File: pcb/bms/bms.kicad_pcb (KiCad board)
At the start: 4 copper layers, 80 x 60 mm, 89 parts, among them J12 Taps 6-8, J13 Taps 0-5, J14 USB_B_Micro, J18 SWD, Q1 FCX495TA, Q2 CSD19506KTT, Q3 CSD19506KTT, Q4 ZXMP10A13FTA, Q5 ZXMP10A13FTA, SW1 Boot, SW2 Wake, SW3 NRST, U1 BQ76942PFBR, U2 STM32L422KBTx

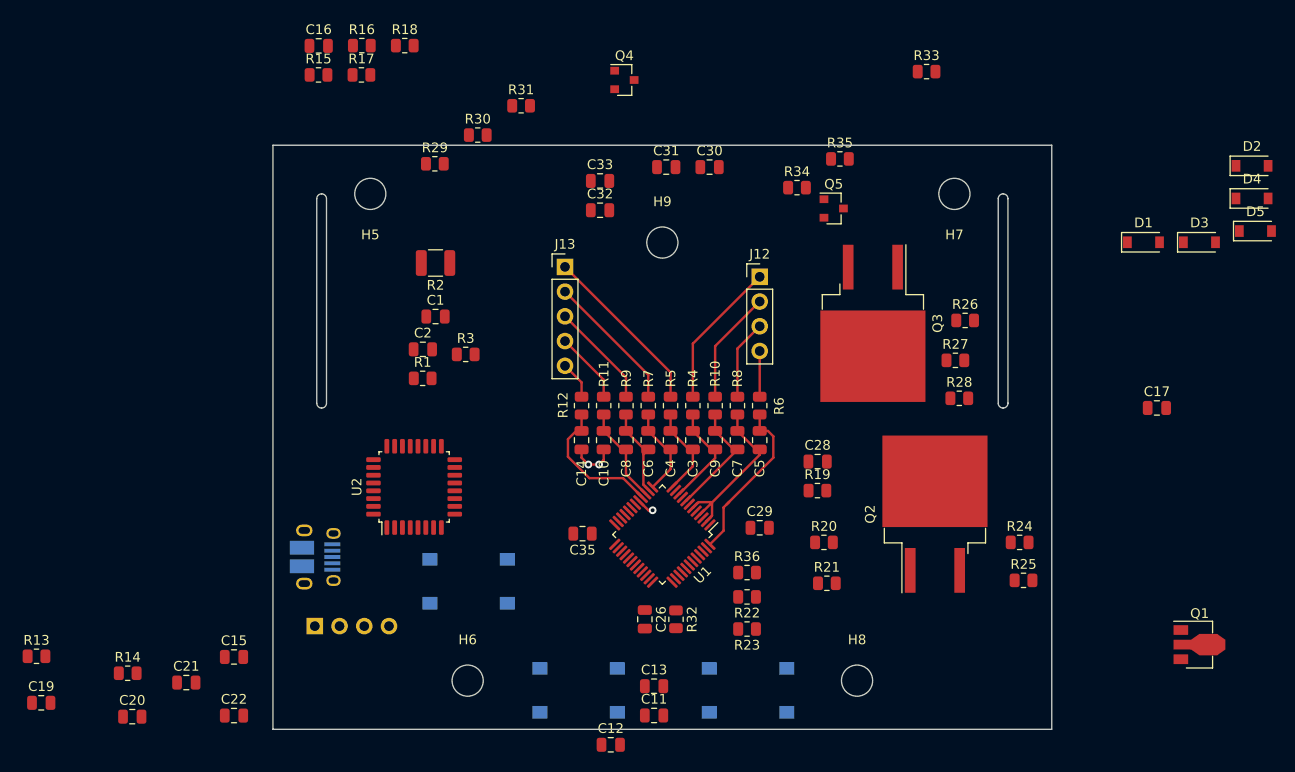
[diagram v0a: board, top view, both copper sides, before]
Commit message: pretty much ready to go
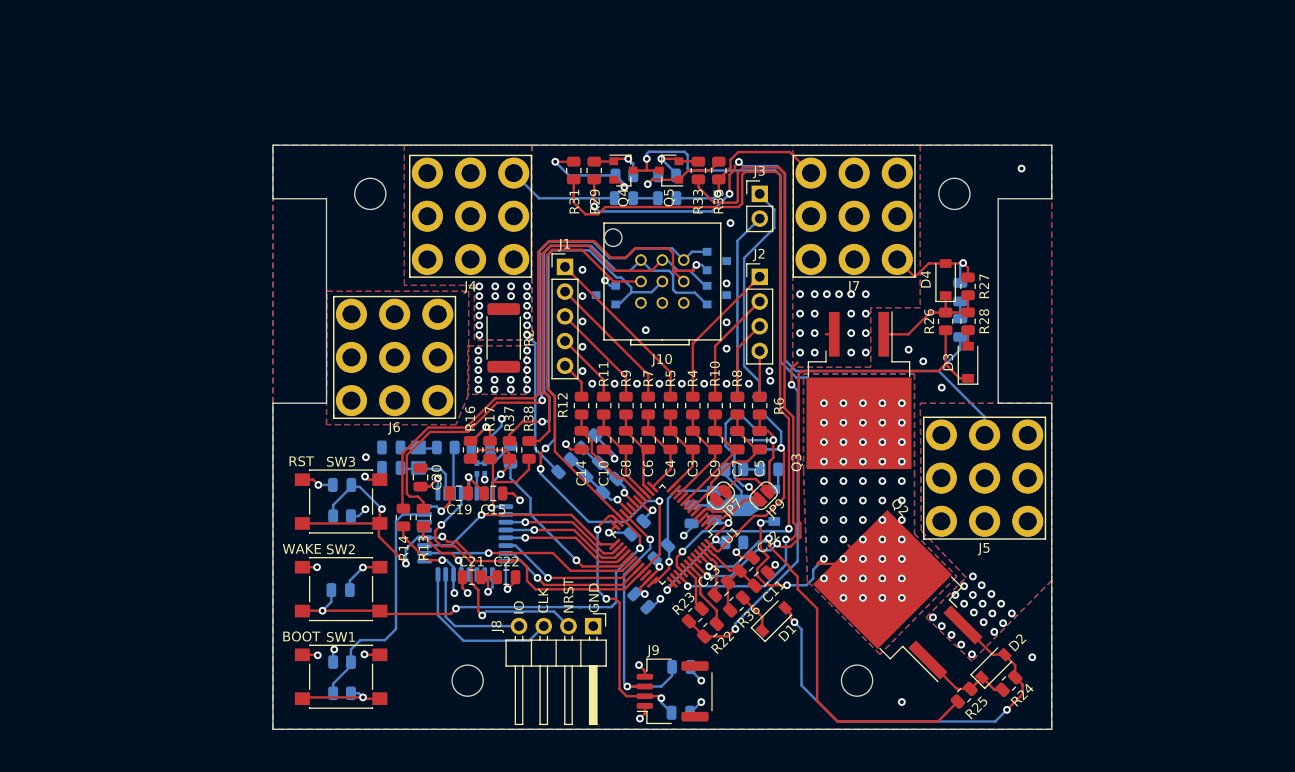
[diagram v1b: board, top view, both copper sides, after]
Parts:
- removed H9: MountingHole, MountingHole:MountingHole_3.2mm_M3
- removed J14: USB_B_Micro, Connect:USB_Micro-B_10103594-0001LF
- removed J18: SWD, Connector_PinHeader_2.54mm:PinHeader_1x04_P2.54mm_Horizontal
- added C18: 100n, Capacitor_SMD:C_0805_2012Metric, B.Cu at (92.0, 113.6)
- added C23: 100n, Capacitor_SMD:C_0805_2012Metric, B.Cu at (91.9, 118.3)
- added C24: 220n, Capacitor_SMD:C_0805_2012Metric, B.Cu at (100.0, 90.3)
- added C25: 220n, Capacitor_SMD:C_0805_2012Metric, B.Cu at (97.7, 90.3)
- added C27: 100n, Capacitor_SMD:C_0805_2012Metric, B.Cu at (71.3, 91.1)
- added C34: 8p, Capacitor_SMD:C_0805_2012Metric, B.Cu at (62.1, 93.2)
- added C36: 8p, Capacitor_SMD:C_0805_2012Metric, B.Cu at (62.1, 91.0)
- added D6: 5.5V, Package_TO_SOT_SMD:SOT-23, B.Cu at (95.6, 71.9)
- added D7: 5.5V, Package_TO_SOT_SMD:SOT-23, B.Cu at (95.6, 75.4)
- added D8: 5.5V, Package_TO_SOT_SMD:SOT-23, B.Cu at (84.2, 75.4)
- added J10: Signals, Connector_Hirose:Hirose_DF62WZ-9P-2.2DSA, F.Cu at (90.0, 74.0)
- added J3: Taps 9-10, Connector_PinHeader_2.54mm:PinHeader_1x02_P2.54mm_Vertical, F.Cu at (100.0, 65.0)
- added J4: Batt- Out, farasis_p10a_pack:74651195R, F.Cu at (70.3, 67.3)
- added J5: Batt+ In, farasis_p10a_pack:74651195R, F.Cu at (123.1, 94.2)
- added J6: Batt- In, farasis_p10a_pack:74651195R, F.Cu at (62.5, 81.8)
- added J7: Batt+ Out, farasis_p10a_pack:74651195R, F.Cu at (109.7, 67.3)
- added J8: SWD, Connector_PinHeader_2.54mm:PinHeader_1x04_P2.54mm_Horizontal, F.Cu at (82.9, 109.4)
- added J9: Thermistors, Connector_JST:JST_NSH_SM04B-NSHSS-TB_1x04-1MP_P1.00mm_Vertical, F.Cu at (88.2, 117.6)
- added JP7: Jumper_NO_Small, Jumper:SolderJumper-2_P1.3mm_Open_RoundedPad1.0x1.5mm, F.Cu at (96.0, 96.0)
- added JP9: Jumper_NO_Small, Jumper:SolderJumper-2_P1.3mm_Open_RoundedPad1.0x1.5mm, F.Cu at (100.4, 96.0)
- added R37: 20, Resistor_SMD:R_0805_2012Metric, F.Cu at (74.3, 91.3)
- added R38: 20, Resistor_SMD:R_0805_2012Metric, F.Cu at (76.3, 91.3)
- added R39: 10k, Resistor_SMD:R_0805_2012Metric, B.Cu at (57.1, 113.1)
- added R40: 20, Resistor_SMD:R_0805_2012Metric, B.Cu at (100.0, 86.8)
- added R41: 20, Resistor_SMD:R_0805_2012Metric, B.Cu at (97.7, 86.8)
- added R42: Rext, Resistor_SMD:R_0805_2012Metric, B.Cu at (67.8, 91.0)
- added X1: ASCO, Oscillator:Oscillator_SMD_Abracon_ASCO-4Pin_1.6x1.2mm, B.Cu at (71.3, 93.2)
- added Y1: 32.768kHz, Crystal:Crystal_SMD_MicroCrystal_CC8V-T1A-2Pin_2.0x1.2mm_HandSoldering, B.Cu at (65.0, 92.1)
- C1, C16, C17, C2, C26, C28, C29, C30, C31, C32, C33, C35, D5, Q1, R1, R15, R18, R19, R20, R21, R3, R30, R32, R34, U2: moved to B.Cu
- R13, R14: value 22 -> 20
- R2: value 2m -> 1m; footprint Resistor_SMD:R_1210_3225Metric -> Resistor_SMD:R_2512_6332Metric
- SW1, SW2: footprint Buttons_Switches_SMD:SW_SPST_PTS645 -> Button_Switch_SMD:SW_SPST_PTS645; moved to F.Cu
- SW3: value NRST -> RST; footprint Buttons_Switches_SMD:SW_SPST_PTS645 -> Button_Switch_SMD:SW_SPST_PTS645; moved to F.Cu
- moved C17 85.9 mm to (57.0, 105.7)
- moved R15 63.6 mm to (57.1, 116.3)
- moved D2 57.8 mm to (124.0, 113.5), turned to 45 degrees
- moved D5 56.9 mm to (101.5, 97.0), turned to 270 degrees
- moved D1 54.2 mm to (101.4, 108.7), turned to 45 degrees
- moved Q1 50.0 mm to (96.8, 97.0)
- moved R19 48.9 mm to (57.1, 98.1)
- moved C19 48.0 mm to (69.1, 95.8)
- moved C16 45.2 mm to (57.1, 94.9)
- moved R18 43.4 mm to (74.4, 91.8), turned to 270 degrees
- moved SW2 43.1 mm to (57.0, 105.6)
- moved R16 43.0 mm to (70.3, 91.3), turned to 270 degrees
- moved R13 42.2 mm to (65.5, 98.2), turned to 270 degrees
- moved R17 40.7 mm to (72.3, 91.3), turned to 270 degrees
- moved C32 38.9 mm to (120.6, 78.8), turned to 270 degrees
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- renumbered J13 to J1, J12 to J2
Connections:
- net /Microcontroller/USART2_RX renamed /Microcontroller/USART2_RX_
- net /Microcontroller/USART2_TX renamed /Microcontroller/USART2_TX_
- net Net-(C17-Pad1) renamed /WAKE
- C16 pad 1: GND -> +3V3
- C16 pad 2: /Cell Measurement/RST_SHUT -> /RST_SHUT
- C5 pad 1: Net-(C5-Pad1) -> Net-(C25-Pad2)
- R14 pad 1: /Microcontroller/USB_DP -> /USB_DP
- R19 pad 1: /Cell Measurement/RST_SHUT -> /RST_SHUT
- R6 pad 2: Net-(C5-Pad1) -> Net-(C25-Pad2)
- SW3 pad 1: GND -> +3V3
- SW3 pad 2: /Cell Measurement/RST_SHUT -> /RST_SHUT
- U1 pad 1: Net-(U1-Pad1) -> (no net)
- U1 pad 11: Net-(U1-Pad11) -> (no net)
- U1 pad 19: Net-(U1-Pad19) -> (no net)
- U1 pad 2: Net-(C5-Pad2) -> Net-(C24-Pad2)
- U1 pad 3: Net-(U1-Pad3) -> (no net)
- U1 pad 33: /Cell Measurement/RST_SHUT -> /RST_SHUT
- U1 pad 34: Net-(U1-Pad34) -> (no net)
- U1 pad 38: Net-(U1-Pad38) -> (no net)
- U1 pad 4: Net-(C5-Pad2) -> Net-(C25-Pad2)
- U1 pad 44: Net-(U1-Pad44) -> (no net)
- U1 pad 48: Net-(C5-Pad1) -> Net-(C24-Pad1)
- U1 pad 5: Net-(U1-Pad5) -> (no net)
- U1 pad 7: Net-(U1-Pad7) -> (no net)
- U1 pad 9: Net-(U1-Pad9) -> (no net)
- U2 pad 14: /Cell Measurement/DDSG -> /Cell Measurement/DCHG
- U2 pad 15: /Cell Measurement/DCHG -> /Cell Measurement/DDSG
- U2 pad 18: Net-(U2-Pad18) -> (no net)
- U2 pad 19: Net-(U2-Pad19) -> (no net)
- U2 pad 2: Net-(U2-Pad2) -> /Microcontroller/OSC_IN
- U2 pad 20: Net-(U2-Pad20) -> (no net)
- U2 pad 25: Net-(U2-Pad25) -> (no net)
- U2 pad 28: /Cell Measurement/RST_SHUT -> /RST_SHUT
- U2 pad 29: Net-(U2-Pad29) -> (no net)
- U2 pad 3: Net-(U2-Pad3) -> /Microcontroller/OSC_OUT
- U2 pad 30: Net-(U2-Pad30) -> (no net)
- U2 pad 4: /Cell Measurement/RST_SHUT -> /Microcontroller/NRST
- U2 pad 6: Net-(U2-Pad6) -> /Microcontroller/HSE
- U2 pad 7: Net-(U2-Pad7) -> (no net)
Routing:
- net BATT+_CONST: track 0.00 -> 119.9 mm, vias 0 -> 25
- net /RST_SHUT: track 0.00 -> 117.0 mm, vias 0 -> 6
- net /WAKE: track 0.00 -> 89.2 mm, vias 0 -> 4
- net /Cell Measurement/PCHG: track 0.00 -> 78.9 mm, vias 0 -> 2
- net /Cell Measurement/CENTER_CHG_DSG: track 0.00 -> 72.6 mm, vias 0 -> 57
- net /Cell Measurement/PDSG: track 0.00 -> 67.7 mm, vias 0 -> 2
- net +BATT: track 0.00 -> 67.1 mm, vias 0 -> 22
- net GND: track 6.50 -> 68.4 mm, vias 3 -> 60
- net /USB_DP: track 0.00 -> 59.9 mm, vias 0 -> 1
- net /Microcontroller/USB_DM: track 0.00 -> 58.0 mm, vias 0 -> 1
- net +3V3: track 0.00 -> 57.4 mm, vias 0 -> 12
- net /Cell Measurement/DSG: track 0.00 -> 52.4 mm, vias 0 -> 2
- net /TX: track 0.00 -> 44.1 mm, vias 0 -> 1
- net /Cell Measurement/CHG: track 0.00 -> 43.9 mm, vias 0 -> 2
- net /RX: track 0.00 -> 41.0 mm
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- added copper zone on B.Cu, net +BATT
- added copper zone on F.Cu, net +BATT
- added copper zone on In1.Cu, net +BATT
- added copper zone on In2.Cu, net +BATT
- added copper zone on B.Cu, net -BATT
- added copper zone on F.Cu, net -BATT
- added copper zone on In1.Cu, net -BATT
- added copper zone on In2.Cu, net -BATT
- added copper zone on B.Cu, net /Cell Measurement/CENTER_CHG_DSG
- added copper zone on F.Cu, net /Cell Measurement/CENTER_CHG_DSG
- added copper zone on In1.Cu, net /Cell Measurement/CENTER_CHG_DSG
- added copper zone on In2.Cu, net /Cell Measurement/CENTER_CHG_DSG
- added copper zone on B.Cu, net BATT+_CONST
- added copper zone on F.Cu, net BATT+_CONST
- added copper zone on In1.Cu, net BATT+_CONST
- added copper zone on In2.Cu, net BATT+_CONST
- added copper zone on B.Cu, net GND
- added copper zone on F.Cu, net GND
- added copper zone on In1.Cu, net GND
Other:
- outline, holes or cut-outs redrawn
- board text added: "BOOT"
- board text added: "CLK"
- board text added: "GND"
- board text added: "IO"
- board text added: "NRST"
- board text added: "RST"
- board text added: "WAKE"
